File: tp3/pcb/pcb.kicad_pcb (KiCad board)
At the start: 2 copper layers, 49.5 x 33.5 mm, 19 parts, among them J1 Screw_Terminal_01x02, J2 Screw_Terminal_01x03, J3 Conn_01x02_Pin, U1 TL084

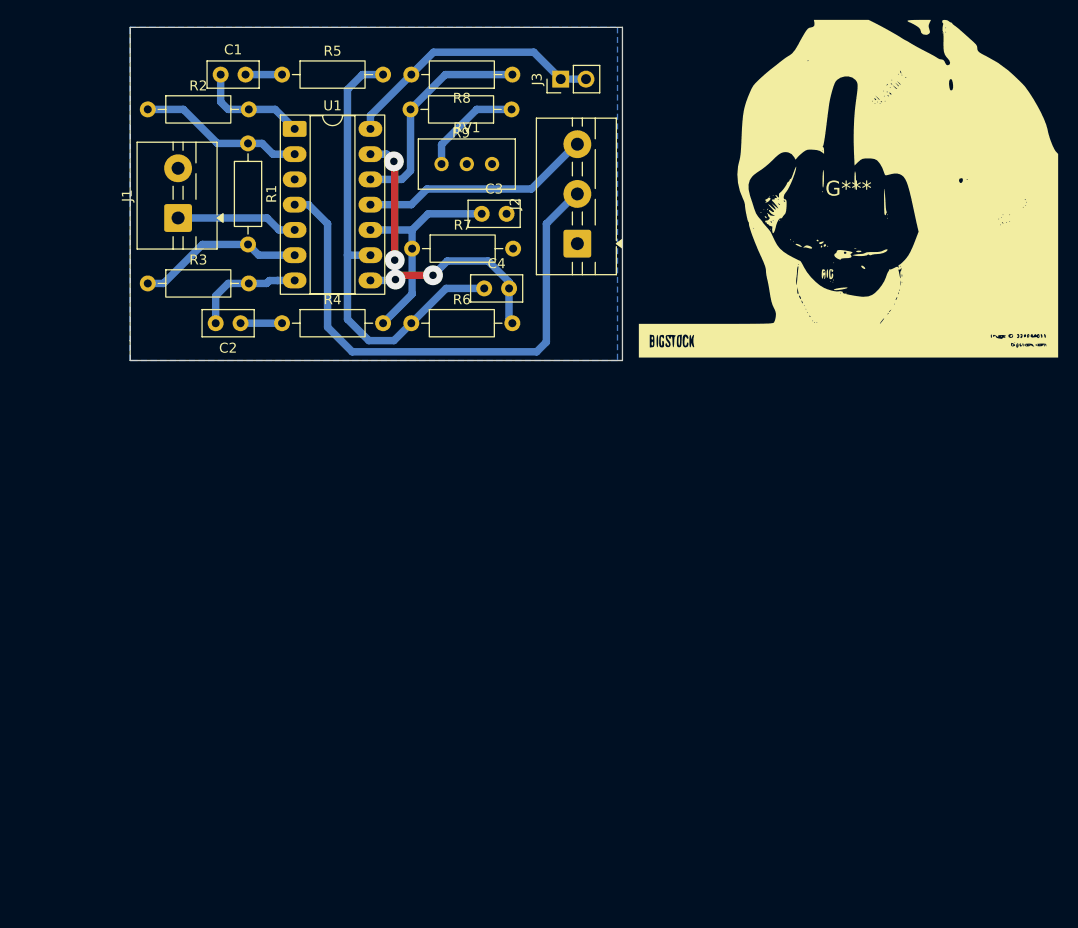
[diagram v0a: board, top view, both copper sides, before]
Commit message: Diseña placa V2
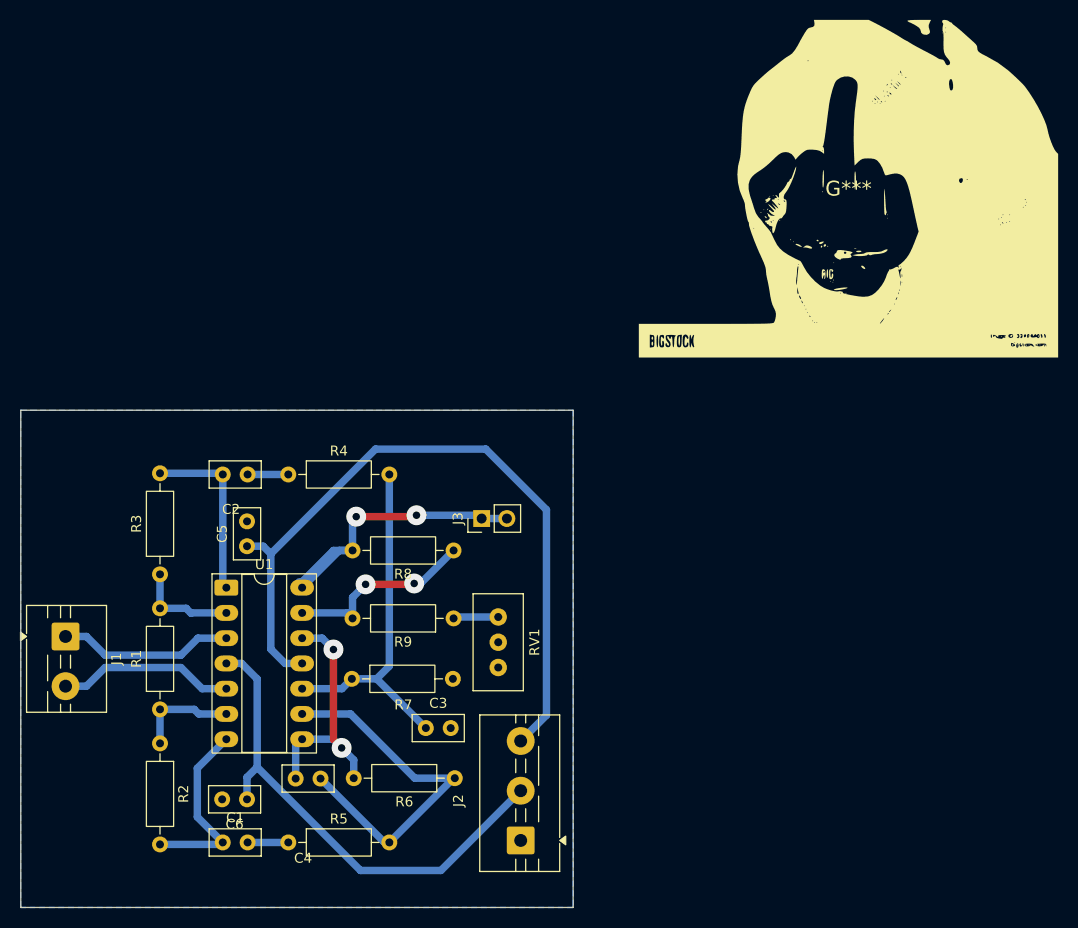
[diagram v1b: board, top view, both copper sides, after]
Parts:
- added C5: 100 nF, Capacitor_THT:C_Disc_D5.0mm_W2.5mm_P2.50mm, F.Cu at (128.8, 121.7)
- added C6: 100 nF, Capacitor_THT:C_Disc_D5.0mm_W2.5mm_P2.50mm, F.Cu at (128.8, 147.1)
- moved R5 77.2 mm to (132.9, 151.5)
- moved C1 77.2 mm to (126.3, 151.5)
- moved R2 63.8 mm to (120.0, 141.5), turned to -90 degrees
- moved J2 60.3 mm to (156.3, 151.3)
- moved R1 57.6 mm to (120.0, 138.1), turned to 90 degrees
- moved C3 52.0 mm to (146.7, 140.0)
- moved C4 52.0 mm to (136.1, 145.0), turned to 180 degrees
- moved R9 51.5 mm to (149.5, 128.9)
- moved RV1 50.6 mm to (154.0, 133.9), turned to -90 degrees
- moved R8 48.2 mm to (149.5, 122.1)
- moved U1 46.6 mm to (126.7, 125.8)
- moved R6 46.0 mm to (149.6, 145.0), turned to 180 degrees
- moved J3 44.9 mm to (152.3, 118.9)
- moved R7 43.7 mm to (139.3, 135.0)
- moved J1 43.6 mm to (110.5, 130.8), turned to -90 degrees
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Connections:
- net /V1 renamed /Vo_N
- net /V2 renamed /Vo_P
- C1 pad 1: Net-(C1-Pad1) -> /V_N
- C2 pad 2: Net-(C2-Pad2) -> /V_P
- J1 pad 1: Net-(J1-Pin_1) -> /Vi_P
- J1 pad 2: GNDREF -> /Vi_N
- R1 pad 1: Net-(U1A--) -> Net-(U1B--)
- R1 pad 2: Net-(U1B--) -> Net-(U1A--)
- R2 pad 1: Net-(U1A--) -> Net-(U1B--)
- R2 pad 2: Net-(C1-Pad1) -> /V_N
- R3 pad 1: Net-(U1B--) -> Net-(U1A--)
- R3 pad 2: Net-(C2-Pad2) -> /V_P
- R8 pad 1: Net-(U1D-+) -> Net-(U1D--)
- R9 pad 2: Net-(U1D-+) -> Net-(U1D--)
- U1 pad 1: Net-(C1-Pad1) -> /V_P
- U1 pad 12: Net-(U1D-+) -> /V_Processed
- U1 pad 13: /V_Processed -> Net-(U1D--)
- U1 pad 3: GNDREF -> /Vi_P
- U1 pad 5: Net-(J1-Pin_1) -> /Vi_N
- U1 pad 7: Net-(C2-Pad2) -> /V_N
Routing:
- net -15V: track 23.2 -> 75.0 mm
- net Net-(U1D-+): track 22.3 -> 0.00 mm
- net Net-(U1D--): track 0.00 -> 19.5 mm, vias 0 -> 2
- net /V_N: track 0.00 -> 19.0 mm
- net /V_P: track 0.00 -> 17.9 mm
- net /Vi_N: track 0.00 -> 17.8 mm
- net /Vi_P: track 0.00 -> 17.7 mm
- net /Vo_P: track 22.5 -> 36.0 mm
- net Net-(J1-Pin_1): track 12.2 -> 0.00 mm
- net Net-(C2-Pad2): track 11.3 -> 0.00 mm
- net Net-(C1-Pad1): track 11.3 -> 0.00 mm
- net /V_Processed: track 34.5 -> 24.8 mm, vias 4 -> 2
- net /Vo_N: track 46.4 -> 36.9 mm
- net Net-(U1B--): track 16.8 -> 10.3 mm
- net Net-(U1A--): track 16.6 -> 10.3 mm
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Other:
- board size 49.5 x 33.5 mm -> 55.5 x 50 mm
